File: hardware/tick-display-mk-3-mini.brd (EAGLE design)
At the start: 59.5 x 33 mm, 18 parts, among them IC1 ATTINY84, IC2 DS1307, IC3 74595DIP, Y1 32.768kHz

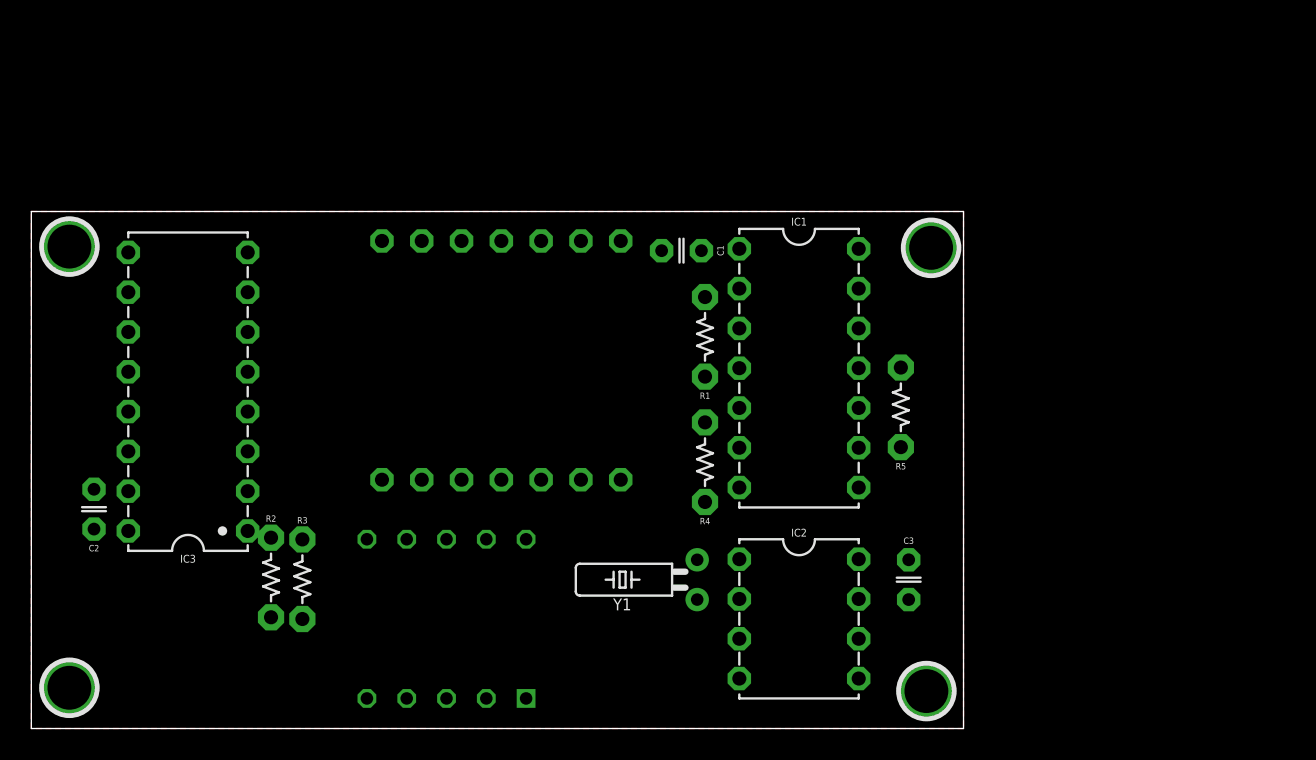
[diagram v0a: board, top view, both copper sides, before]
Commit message: scaled down even more
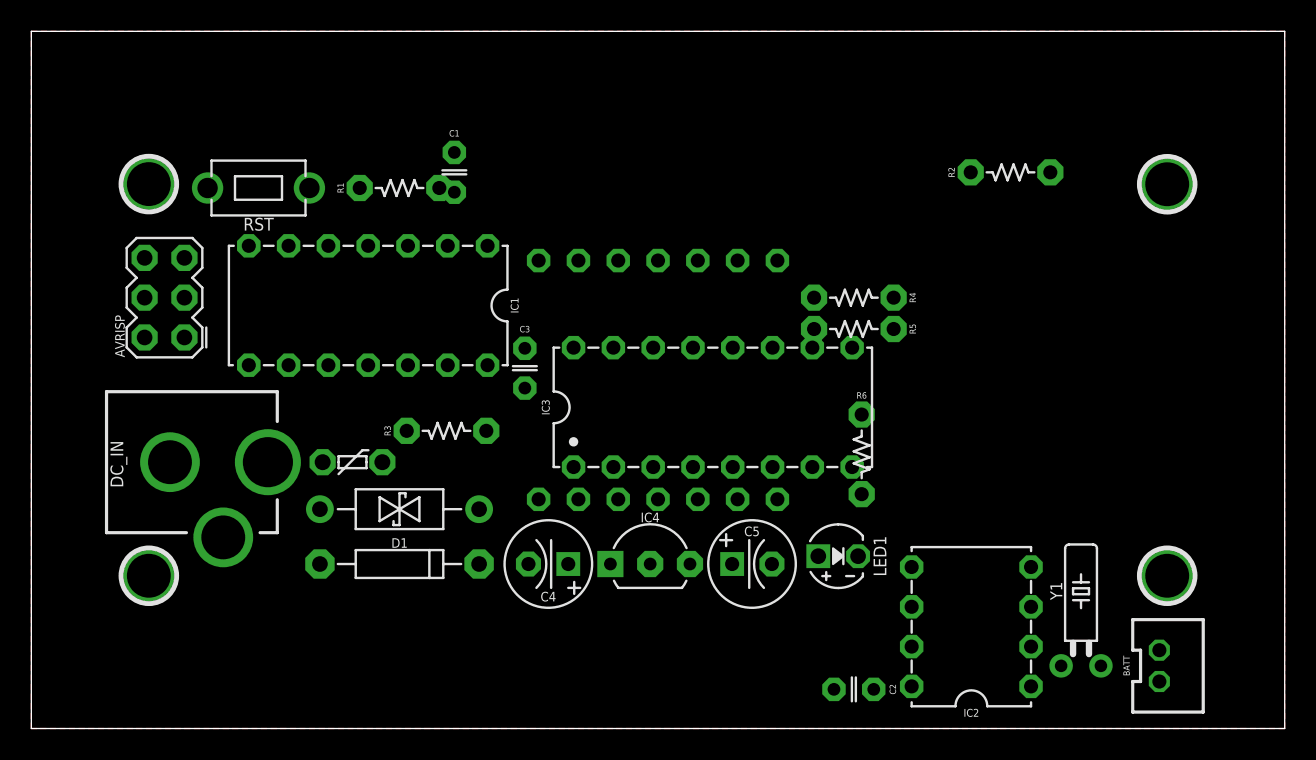
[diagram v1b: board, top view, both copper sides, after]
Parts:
- removed TEMP_C: 7SEG_2DIG, A_butts:7SEG_2DIG_14MM
- removed TIME: 7SED_4DIGIT_14MM14.2MM-CC, A_butts:7SEG_4DIG
- added AVRISP: AVR_SPI_PRG_6PTH, A_butts:2X3
- added BATT: M02JST-PTH-VERT, A_butts:JST-2-PH-VERT-PTH
- added C4: 10uF, A_butts:E2,5-6
- added C5: 100uF, A_butts:E2,5-6
- added D1: 1N5819, A_butts:DIODE-10.16MM
- added DC_IN: (no value), A_butts:DCJACK_2MM_PTH
- added DISPLAY: 7SED_4DIGIT_14MM14.2MM-CC, A_butts:7SEG_4DIG
- added F1: PTCPTH, A_butts:PTC
- added IC4: LM2931, A_butts:TO-92-AMMO
- added LED1: LED3MM, A_butts:LED3MM
- added R6: 330R, A_butts:RESISTOR-AXIAL-PTH-5.08MM
- added RST: SPST-NO-TACT3MM-PTH-SMALL-PADS, A_butts:DTS-3-SMALL-PADS
- added TVS1: (no value), A_butts:DO-41-TVS
- IC3: value 74595DIP -> 74HCT595
- moved R2 53.8 mm to (62.5, 35.5), turned to 0 degrees
- moved C2 49.8 mm to (52.5, 2.50), turned to 180 degrees
- moved IC3 33.5 mm to (43.5, 20.5), turned to 0 degrees
- moved C3 28.0 mm to (31.5, 23.0)
- moved IC1 27.8 mm to (21.5, 27.0), turned to 180 degrees
- moved Y1 25.1 mm to (67.0, 4.00), turned to 0 degrees
- moved R1 21.7 mm to (23.5, 34.5), turned to 0 degrees
- moved H1 17.0 mm to (72.5, 9.75)
- moved H3 15.6 mm to (72.5, 34.7)
- moved C1 15.3 mm to (27.0, 35.5), turned to 270 degrees
- moved R4 14.2 mm to (52.5, 27.5), turned to 180 degrees
- moved R3 13.2 mm to (26.5, 19.0), turned to 0 degrees
- moved IC2 11.0 mm to (60.0, 6.50), turned to 90 degrees
- moved H4 8.77 mm to (7.50, 9.75)
- moved H2 6.45 mm to (7.50, 34.8)
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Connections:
- removed net TC1: IC1.12, TEMP_C.5
- removed net TC2: IC1.13, TEMP_C.10
- removed net VBAT: IC2.3
- new net DP: DISPLAY.P$3, IC3.7
- new net MISO: AVRISP.1, IC1.8
- new net N$1: BATT.1, IC2.3
- new net N$10: LED1.A, R6.P$2
- new net N$3: DC_IN.PWR, F1.P$1
- new net N$5: C4.+, D1.C, IC4.1
- new net RESET: AVRISP.5, IC1.4, R1.P$1, RST.1
- net A: now also DISPLAY.P$13; no longer TEMP_C.4, TIME.P$13
- net B: now also DISPLAY.P$9; no longer TEMP_C.3, TIME.P$9
- net C: now also DISPLAY.P$4; no longer TEMP_C.9, TIME.P$4
- net D: now also DISPLAY.P$2; no longer TEMP_C.8, TIME.P$2
- net E: now also DISPLAY.P$1; no longer TEMP_C.6, TIME.P$1
- net F: now also DISPLAY.P$12; no longer TEMP_C.7, TIME.P$12
- net G: now also DISPLAY.P$5; no longer TEMP_C.1, TIME.P$5
- net GND: now also AVRISP.6, BATT.2, C4.-, C5.-, DC_IN.BRK, DC_IN.GND, DISPLAY.P$7, IC4.2, LED1.K, RST.2, TVS1.P$1; no longer TIME.P$7
- net HR1: now also DISPLAY.P$14, IC1.10; no longer IC1.6, TIME.P$14
- net HR2: now also DISPLAY.P$11, IC1.11; no longer IC1.8, TIME.P$11
- net MI1: now also DISPLAY.P$10, IC1.12; no longer IC1.10, TIME.P$10
- net MI2: now also DISPLAY.P$6, IC1.13; no longer IC1.11, TIME.P$6
- net N$18: now also DISPLAY.P$8; no longer TIME.P$8
- net N$4: now also D1.A, F1.P$2, TVS1.P$2; no longer IC1.4, R1.P$1
- net SCL: now also AVRISP.3
- net SDA: now also AVRISP.4
- net VCC: now also AVRISP.2, C5.+, IC4.3, R6.P$1
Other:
- board size 59.5 x 33 mm -> 80 x 44.5 mm

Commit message: again with the not sure what the fuck i was thinking
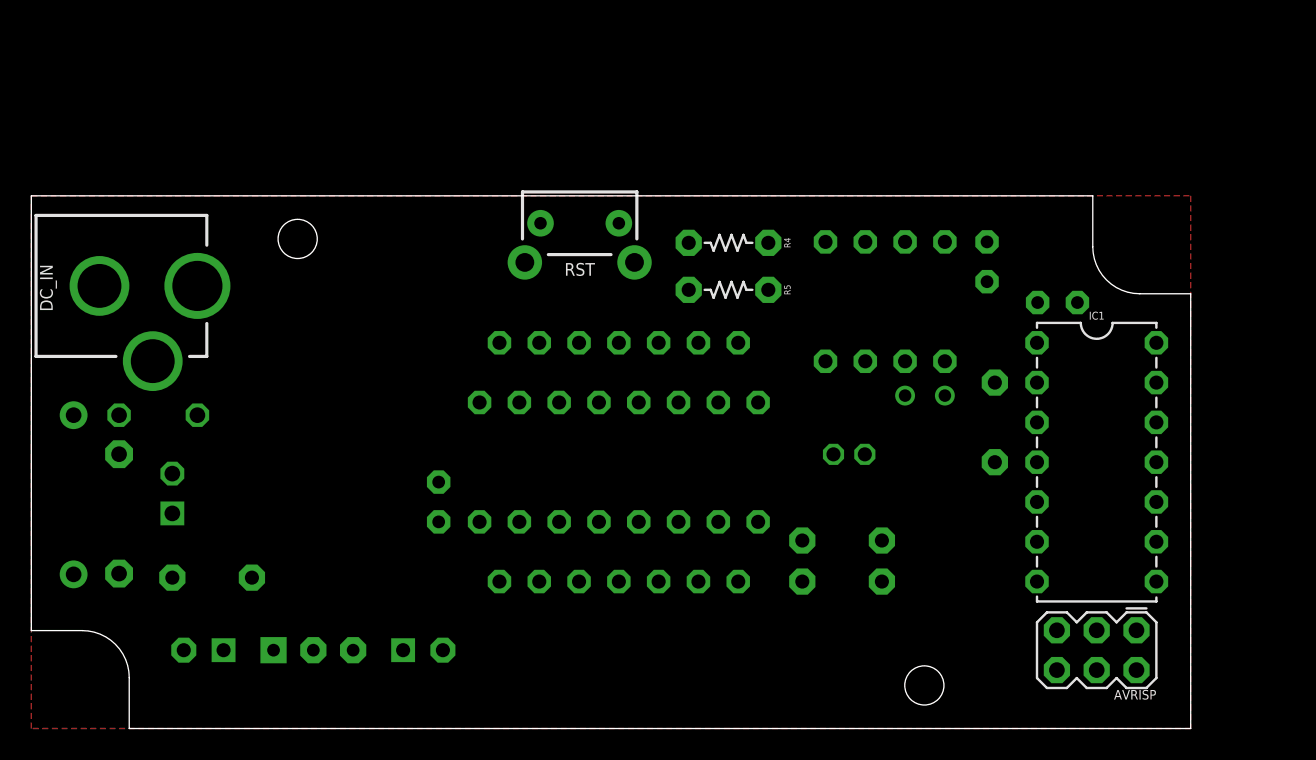
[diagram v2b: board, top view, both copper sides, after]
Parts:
- removed H1, H2, H3, H4: HOLE#2, A_butts:HOLE-#2
- D1: device A_butts:DIODE-10.16MM -> A_butts:DIODE-7.68MM
- DISPLAY: value 7SED_4DIGIT_14MM14.2MM-CC -> 7SED_4DIGIT_14MM14.2MM-CC-NS; device A_butts:7SEG_4DIG -> A_butts:7SEG_4DIG_NS
- RST: value SPST-NO-TACT3MM-PTH-SMALL-PADS -> SPST-NO-TACT3MM-RA; device A_butts:DTS-3-SMALL-PADS -> A_butts:TACTILE-PTH-SIDE
- moved AVRISP 63.6 mm to (68.0, 5.00), turned to 180 degrees
- moved IC1 47.6 mm to (68.0, 17.0), turned to 270 degrees
- moved LED1 42.7 mm to (9.00, 15.0), flipped to the bottom, turned to 90 degrees
- moved R6 42.2 mm to (11.5, 9.63), flipped to the bottom, turned to 0 degrees
- moved R1 40.8 mm to (61.5, 19.5), flipped to the bottom, turned to 90 degrees
- moved C1 39.4 mm to (65.5, 27.2), flipped to the bottom, turned to 180 degrees
- moved C2 28.6 mm to (61.0, 29.8), flipped to the bottom, turned to 270 degrees
- moved R3 27.0 mm to (51.8, 9.38), flipped to the bottom, turned to 180 degrees
- moved R2 25.8 mm to (51.8, 12.0), flipped to the bottom, turned to 180 degrees
- moved BATT 24.0 mm to (52.2, 17.5), flipped to the bottom, turned to 0 degrees
- moved C4 22.7 mm to (11.0, 5.00), flipped to the bottom, turned to 0 degrees
- moved IC4 22.2 mm to (18.0, 5.00), flipped to the bottom, turned to 180 degrees
- moved C5 21.7 mm to (25.0, 5.00), flipped to the bottom, turned to 180 degrees
- moved IC2 21.5 mm to (54.5, 27.2), flipped to the bottom, turned to 0 degrees
- moved TVS1 20.8 mm to (2.70, 14.9), flipped to the bottom, turned to 90 degrees
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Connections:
- net B: now also IC3.7; no longer IC3.1
- net C: now also IC3.4; no longer IC3.2
- net D: now also IC3.2; no longer IC3.3
- net DP: now also IC3.3; no longer IC3.7
- net E: now also IC3.1; no longer IC3.4
- net F: now also IC3.6; no longer IC3.5
- net G: now also IC3.5; no longer IC3.6
- net N$5: now also D1.K; no longer D1.C
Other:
- board size 80 x 44.5 mm -> 74 x 34 mm
